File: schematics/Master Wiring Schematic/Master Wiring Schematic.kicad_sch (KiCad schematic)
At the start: 6 parts, among them J1 M5_Ring_Terminals, J2 Raspberry_Pi_4, J3 UBEC_5V_3A

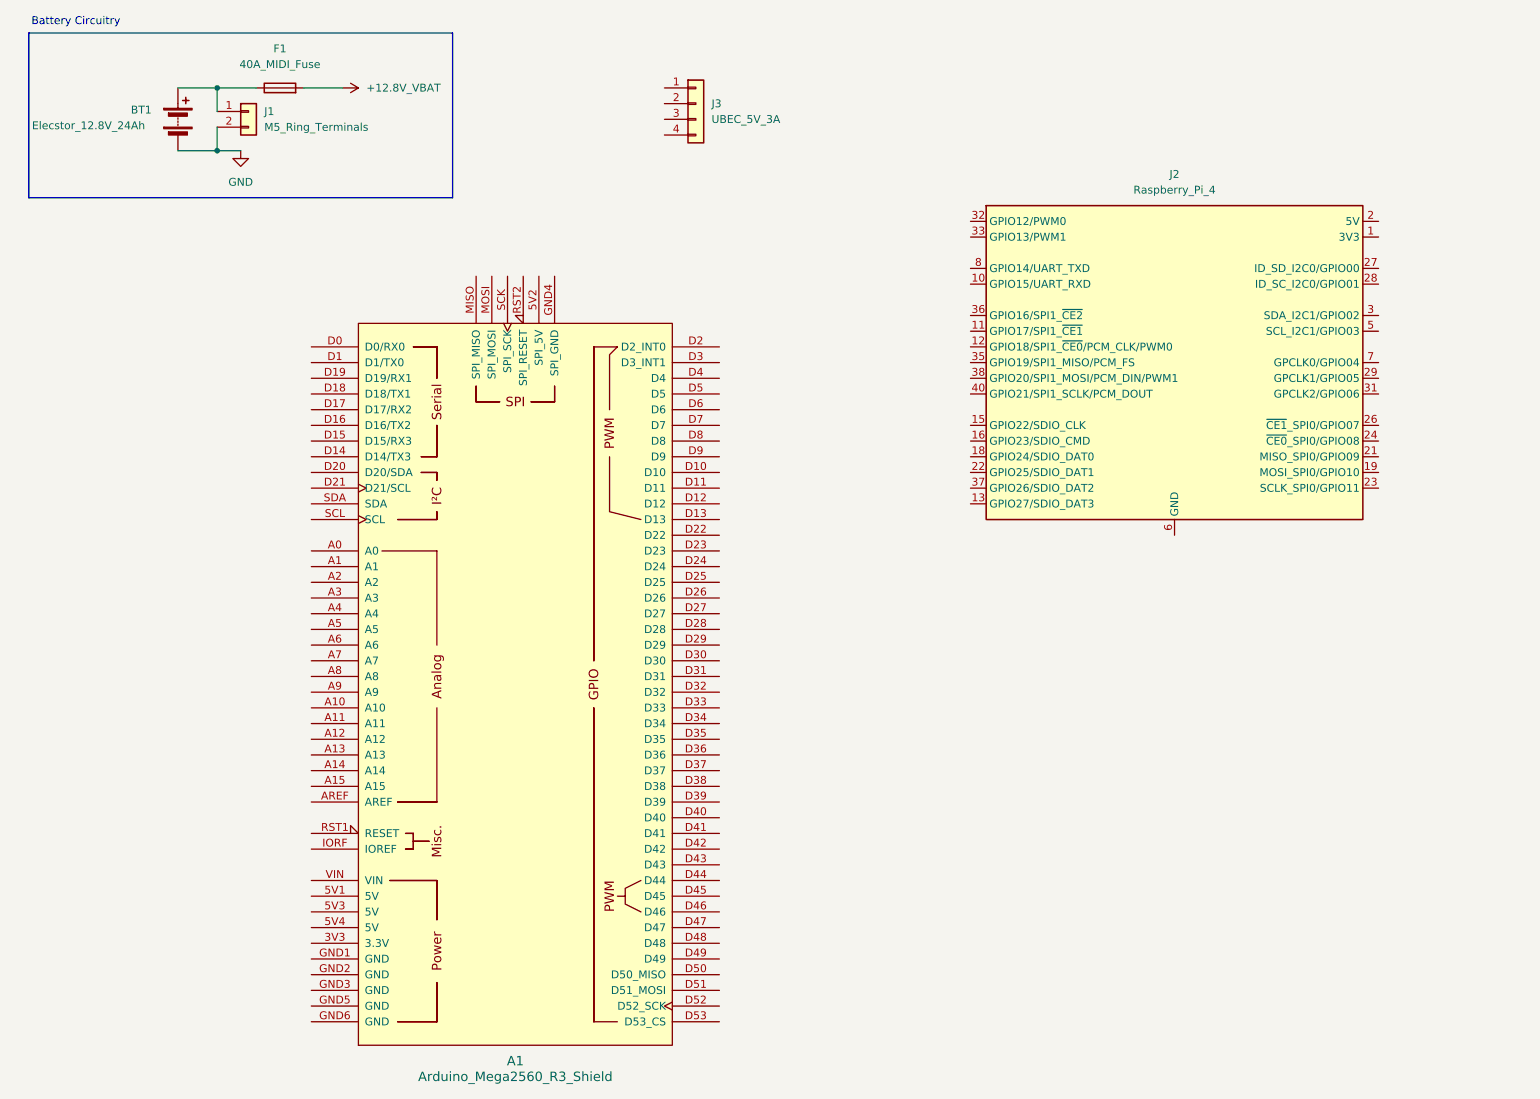
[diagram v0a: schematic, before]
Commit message: Powering the Brains of the Rover
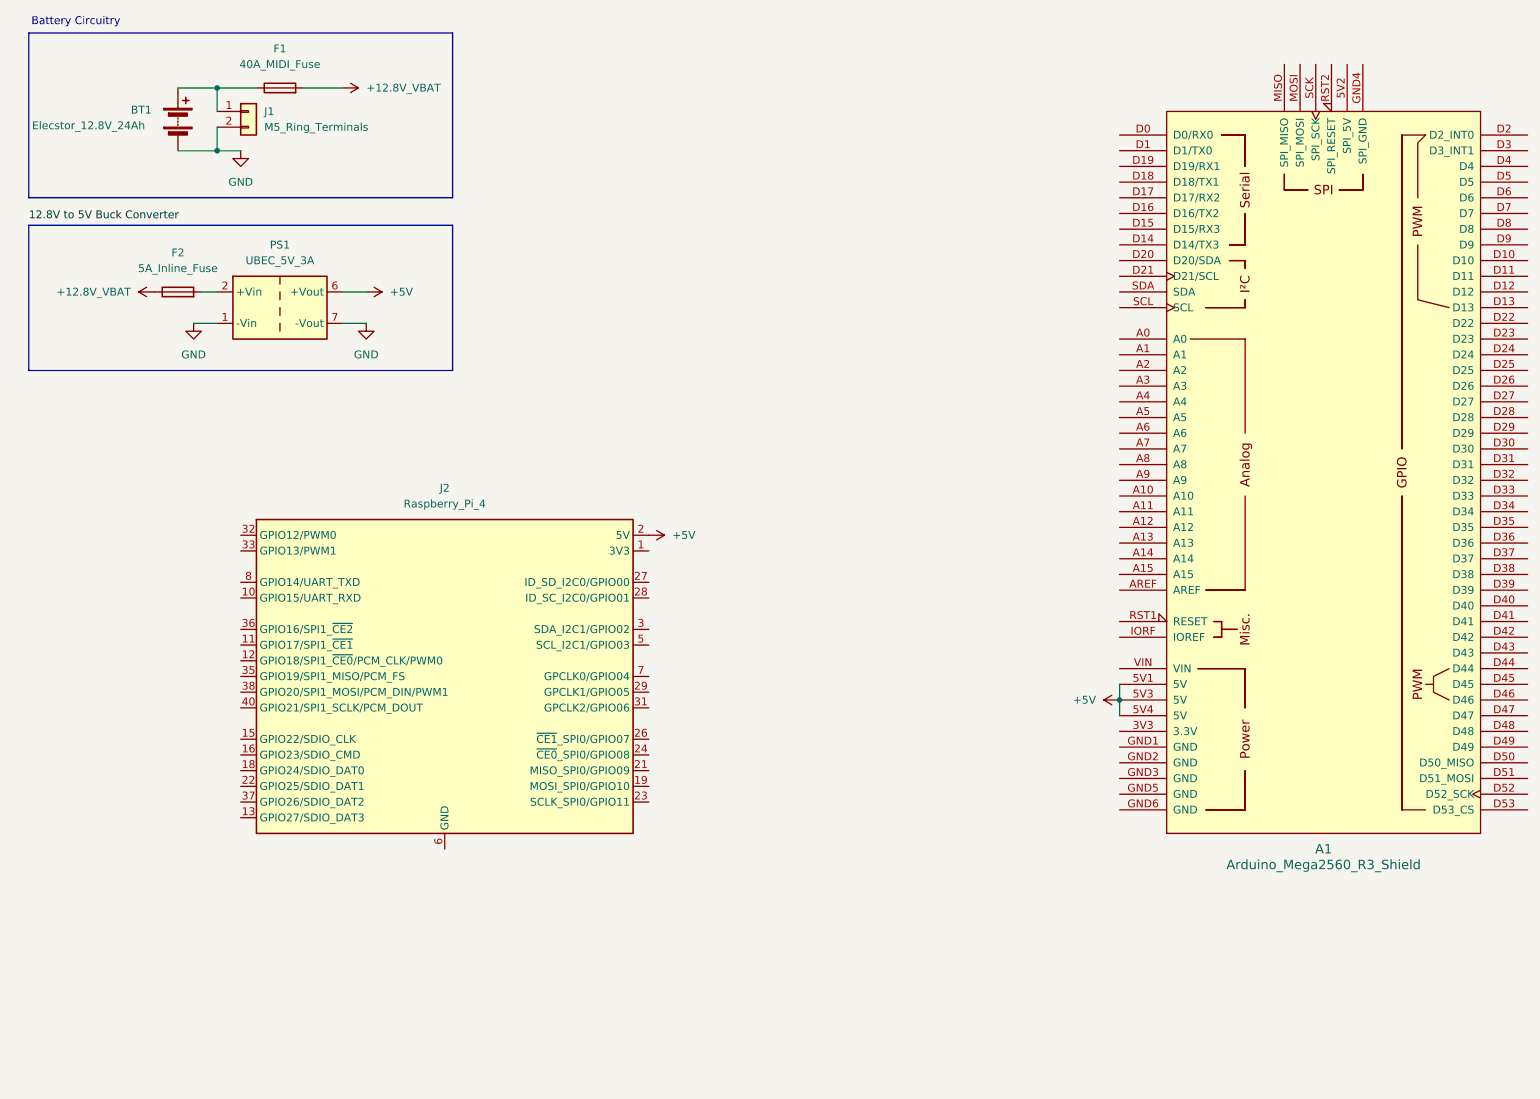
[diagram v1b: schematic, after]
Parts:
- removed J3: UBEC_5V_3A, symbol Connector_Generic:Conn_01x04
- added F2: 5A_Inline_Fuse, symbol Device:Fuse
- added PS1: UBEC_5V_3A, Converter_DCDC:Converter_DCDC_XP_POWER-ITXxxxxSA_THT, symbol Converter_DCDC:ITX1209SA
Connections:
- net +12.8V_VBAT: now also F2.1
- net GND: now also PS1.1 (-Vin), PS1.7 (-Vout)
- net +5V: now reaches A1.5V1 (5V)
- net +5V: now also A1.5V3 (5V), A1.5V4 (5V), J2.2 (5V), J2.4 (5V), PS1.6 (+Vout)
- new net: F2.2, PS1.2 (+Vin)
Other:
- company: (none) -> UCT Space and Astronomy Society
- title: (none) -> Cars4Mars Master Schematic
- moved on the sheet: A1, J2
